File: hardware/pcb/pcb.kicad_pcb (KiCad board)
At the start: 4 copper layers, 41.5 x 61.7 mm, 283 parts, among them J100 Conn_02x05_Odd_Even, J200 Conn_02x05_Odd_Even, J400 AudioJack3_SwitchT, J500 AXT524124, J800 USB_C_Receptacle, SW600 K1-1511SA-02, U1 AXP209, U100 MIMXRT1176DVMAA, U2 SY8008, U200 XC7S25-CSGA225, U201 74LVCH245A, U3 NX3P1108UK, U300 IS66WVC4M16-ALL, U301 MT48H16M32LFB5-6 or IS42VM321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, U302 74LVC1G126, U303 IS66WVC4M16-ALL, U304 74LVC1G126, U4 NX3P1108UK, U400 CS43130, U401 ADP150-1.8, U402 ADP150-1.8, U5 NX3P1108UK, U500 LT3491, U6 NX3P1108UK, U7 ADP121-1.2, U700 W25Q128JVP, U800 USBLC6-2P6, U801 FUSB302UCX, U802 CBTL08GP053, U803 TC358777, X800 19.2MHz, Y100 24MHz, Y101 32.768K, Y400 22.5792MHz

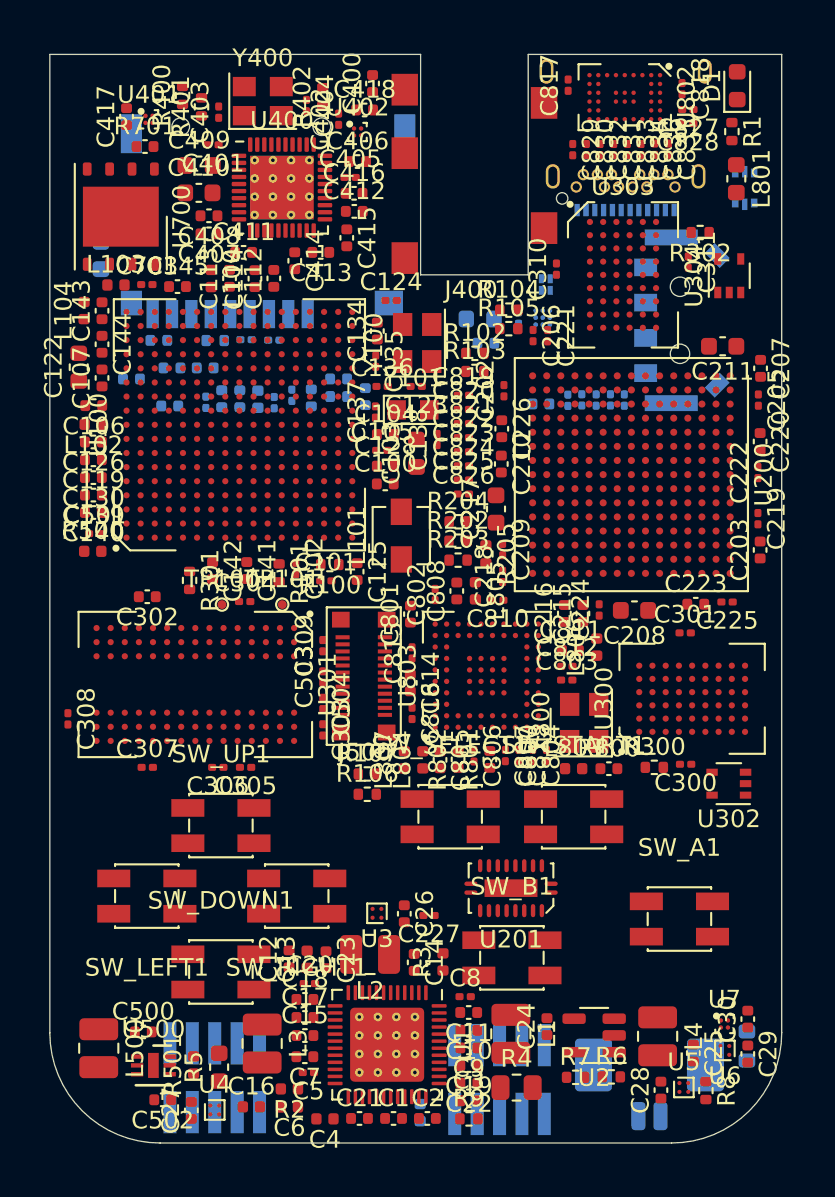
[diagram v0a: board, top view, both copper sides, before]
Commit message: - Working on pcb layout
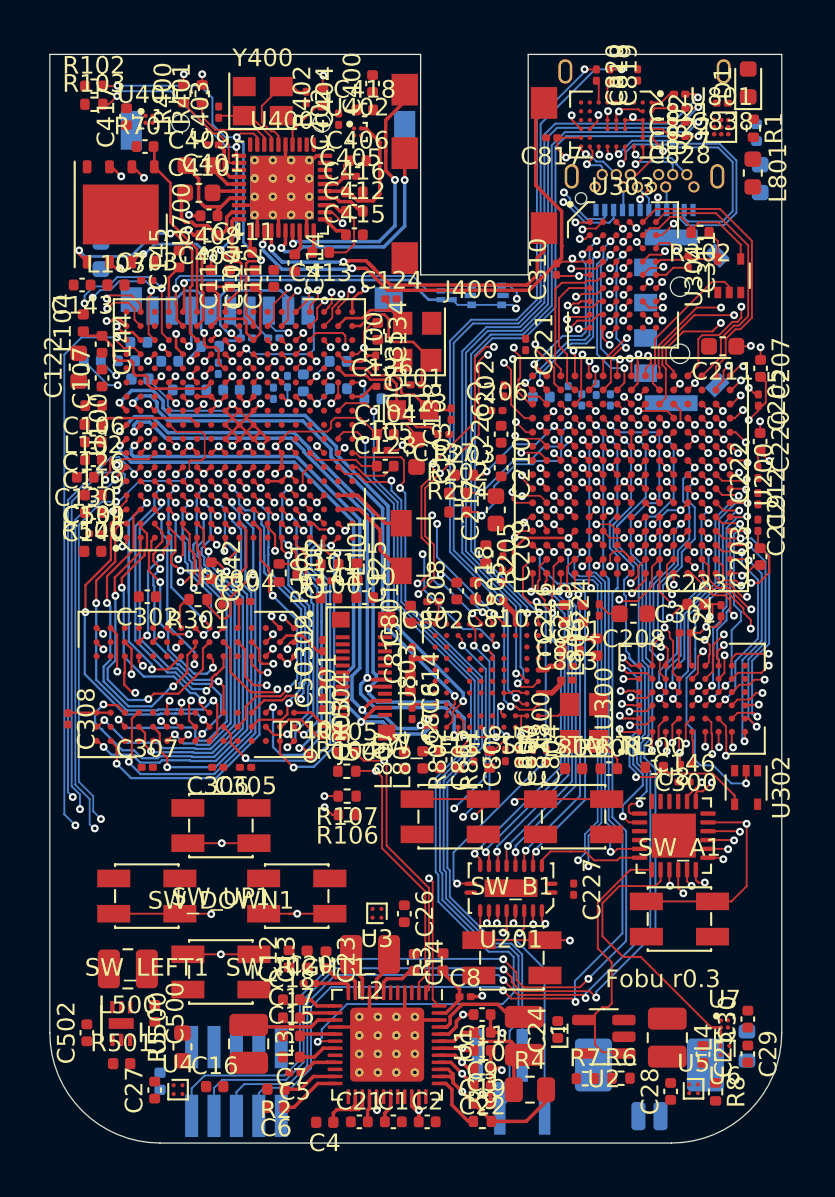
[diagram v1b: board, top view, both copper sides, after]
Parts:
- removed C823, C824, C825, C826, C829, C830, C831, C832, C833, C834, C835, C836: 100nF, Capacitor_SMD:C_0201_0603Metric
- removed J100: Conn_02x05_Odd_Even, Connector_PinHeader_1.27mm:PinHeader_2x05_P1.27mm_Vertical_SMD
- added C146: 100nF, Capacitor_SMD:C_0201_0603Metric, F.Cu at (136.0, 96.0)
- added J101: Conn_01x04, Connector_PinHeader_1.27mm:PinHeader_1x04_P1.27mm_Vertical_SMD_Pin1Left, B.Cu at (126.2, 113.0)
- added U8: PCA9555AHF, Package_DFN_QFN:HVQFN-24-1EP_4x4mm_P0.5mm_EP2.5x2.5mm, F.Cu at (135.4, 99.1)
- C212, C838, U801: moved to F.Cu
- moved R104 27.7 mm to (116.8, 95.4)
- moved R103 26.4 mm to (102.5, 57.6)
- moved R102 26.4 mm to (102.5, 56.6)
- moved R105 25.7 mm to (116.8, 94.4)
- moved C821 22.3 mm to (135.7, 57.0), turned to 180 degrees
- moved C822 22.3 mm to (135.7, 57.8), turned to 180 degrees
- moved C820 20.4 mm to (131.0, 56.0), turned to -90 degrees
- moved C819 20.0 mm to (131.8, 56.0), turned to -90 degrees
- moved C837 19.4 mm to (140.1, 59.2), turned to 90 degrees
- moved L802 17.8 mm to (140.3, 61.8), turned to -90 degrees
- moved C838 16.8 mm to (138.1, 57.5), turned to 180 degrees
- moved U800 15.8 mm to (124.8, 68.4), turned to 0 degrees
- moved J200 14.9 mm to (110.6, 113.0)
- moved R200 14.9 mm to (106.2, 113.0), turned to -90 degrees
- moved U801 14.8 mm to (138.1, 58.9), turned to 0 degrees
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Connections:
- C817 pad 1: +1V8 -> +3V3
- R400 pad 2: SAI4_TX_DATA -> SAI1_RX_SYNC
- R401 pad 2: SAI4_TX_SYNC -> SAI1_RX_BCLK
- R402 pad 2: SAI4_TX_BCLK -> SAI1_RX_DATA0
- U1 pad 6: PMU_VBUSEN -> unconnected-(U1-Pad6)
- U100 pad R5: /mcu/JTAG_TRSTB -> unconnected-(U100-PadR5)
- U100 pad T5: /mcu/JTAG_TDO -> unconnected-(U100-PadT5)
- U100 pad U5: /mcu/JTAG_TDI -> unconnected-(U100-PadU5)
- U200 pad A10: CRAMA_OEN -> CRAMA_A17
- U200 pad A11: CRAMA_CRE -> CRAMA_A15
- U200 pad A12: CRAMA_WAIT -> CRAMA_A13
- U200 pad A14: CRAMA_ADVN -> CRAMA_WAIT
- U200 pad A2: CRAMB_DQ4 -> CRAMB_DQ1
- U200 pad A3: CRAMB_DQ2 -> CRAMB_DQ3
- U200 pad A4: CRAMB_DQ1 -> CRAMB_DQ4
- U200 pad A5: CRAMA_DQ9 -> CRAMA_A20
- U200 pad A6: CRAMA_DQ10 -> CRAMA_A11
- U200 pad A7: CRAMA_DQ6 -> CRAMA_A10
- U200 pad A8: CRAMA_DQ11 -> CRAMA_A9
- U200 pad A9: CRAMA_DQ12 -> CRAMA_ADVN
- U200 pad B1: CRAMB_DQ8 -> CRAMB_A2
- U200 pad B10: CRAMA_LBN -> CRAMA_CEN
- U200 pad B11: CRAMA_CEN -> CRAMA_A14
- U200 pad B12: CRAMA_WEN -> CRAMA_A8
- U200 pad B13: CRAMA_A0 -> CRAMA_A12
- U200 pad B14: CRAMA_A1 -> CRAMA_DQ13
- U200 pad B15: CRAMA_A3 -> CRAMA_DQ15
- U200 pad B2: CRAMB_DQ3 -> CRAMB_DQ2
- U200 pad B5: CRAMB_DQ10 -> CRAMB_DQ7
- U200 pad B9: CRAMA_UBN -> CRAMA_A7
- U200 pad C1: CRAMB_DQ7 -> CRAMB_CRE
- U200 pad C10: CRAMA_DQ15 -> CRAMA_A6
- U200 pad C13: CRAMA_A4 -> CRAMA_A5
- U200 pad C14: CRAMA_A5 -> CRAMA_A19
- U200 pad C15: CRAMA_A2 -> CRAMA_A18
- U200 pad C4: CRAMB_DQ14 -> CRAMB_WEN
- U200 pad C5: CRAMB_DQ9 -> CRAMB_CLK
- U200 pad C6: CRAMA_DQ1 -> CRAMA_DQ7
- U200 pad C7: CRAMA_DQ2 -> CRAMA_WEN
- U200 pad C8: CRAMA_DQ7 -> CRAMA_DQ6
- U200 pad C9: CRAMA_DQ8 -> CRAMA_DQ4
- U200 pad D1: CRAMB_DQ12 -> CRAMB_A0
- U200 pad D10: CRAMA_DQ14 -> CRAMA_DQ1
- U200 pad D11: CRAMA_DQ0 -> CRAMA_DQ2
- U200 pad D12: CRAMA_A6 -> CRAMA_UBN
- U200 pad D13: CRAMA_A7 -> CRAMA_A21
- U200 pad D15: CRAMA_A13 -> CRAMA_DQ14
- U200 pad D2: CRAMB_DQ11 -> CRAMB_A20
- U200 pad D3: CRAMB_OEN -> unconnected-(U200-PadD3)
- U200 pad D4: CRAMB_DQ13 -> CRAMB_ADVN
- U200 pad D7: CRAMA_DQ3 -> CRAMA_DQ0
- U200 pad D8: CRAMA_DQ4 -> CRAMA_DQ3
- U200 pad D9: CRAMA_DQ13 -> CRAMA_A16
- U200 pad E1: CRAMB_LBN -> CRAMB_A1
- U200 pad E11: CRAMA_A9 -> CRAMA_OEN
- U200 pad E12: CRAMA_A10 -> CRAMA_A3
- U200 pad E13: CRAMA_A11 -> CRAMA_A0
- U200 pad E14: CRAMA_A12 -> CRAMA_DQ11
- U200 pad E15: CRAMA_A17 -> CRAMA_DQ12
- U200 pad E2: CRAMB_DQ15 -> CRAMB_A11
- U200 pad E3: CRAMB_UBN -> CRAMB_A10
- U200 pad F1: CRAMB_WEN -> CRAMB_A4
- U200 pad F11: CRAMA_A8 -> CRAMA_A4
- U200 pad F14: CRAMA_A16 -> CRAMA_DQ8
- U200 pad F15: CRAMA_A15 -> CRAMA_DQ9
- U200 pad F3: CRAMB_WAIT -> CRAMB_DQ0
- U200 pad F4: CRAMB_CRE -> CRAMB_A9
- U200 pad G1: CRAMB_ADVN -> CRAMB_A7
- U200 pad G11: CRAMA_A20 -> CRAMA_CRE
- U200 pad G12: CRAMA_A21 -> CRAMA_A1
- U200 pad G13: CRAMA_A18 -> CRAMA_A2
- U200 pad G14: CRAMA_A19 -> CRAMA_DQ10
- U200 pad G15: CRAMA_A14 -> CRAMA_LBN
- U200 pad G4: CRAMB_DQ0 -> CRAMB_WAIT
- U200 pad H1: CRAMB_CLK -> CRAMB_A16
- U200 pad H2: CRAMB_A3 -> CRAMB_A17
- U200 pad H3: CRAMB_A1 -> CRAMB_A8
- U200 pad H4: CRAMB_A0 -> CRAMB_A18
- U200 pad J1: CRAMB_A7 -> CRAMB_A5
- U200 pad J2: CRAMB_A2 -> CRAMB_A3
- U200 pad J3: CRAMB_A5 -> CRAMB_A19
- U200 pad J4: CRAMB_A4 -> CRAMB_DQ15
- U200 pad K1: CRAMB_A6 -> CRAMB_A21
- U200 pad K14: unconnected-(U200-PadK14) -> SAI4_TX_BCLK
- U200 pad K2: CRAMB_A9 -> CRAMB_A6
- U200 pad K3: CRAMB_A8 -> unconnected-(U200-PadK3)
- U200 pad L1: CRAMB_A11 -> CRAMB_A13
- U200 pad L14: unconnected-(U200-PadL14) -> SAI4_TX_SYNC
- U200 pad L15: unconnected-(U200-PadL15) -> SAI4_TX_DATA
- U200 pad M1: CRAMB_A10 -> CRAMB_A15
- U200 pad M10: CSI_D1 -> CSI_D8
- U200 pad M13: unconnected-(U200-PadM13) -> UART2_RXD
- U200 pad M14: /fpga/K_UP -> /fpga/K_RIGHT
- U200 pad M2: CRAMB_A15 -> CRAMB_DQ14
- U200 pad M3: CRAMB_A13 -> CRAMB_A12
- U200 pad M4: CRAMB_A12 -> CRAMB_DQ13
- U200 pad M8: CSI_D13 -> CSI_D10
- U200 pad M9: CSI_D0 -> CSI_D6
- U200 pad N1: CRAMB_A19 -> CRAMB_DQ12
- U200 pad N10: CSI_D4 -> CSI_VSYNC
- U200 pad N11: CSI_D5 -> CSI_D15
- U200 pad N12: CSI_D2 -> CSI_D5
- U200 pad N13: unconnected-(U200-PadN13) -> UART2_TXD
- U200 pad N14: /fpga/K_RIGHT -> /fpga/K_SELECT
- U200 pad N15: /fpga/K_DOWN -> /fpga/K_UP
- U200 pad N2: CRAMB_A14 -> CRAMB_DQ11
- U200 pad N3: CRAMB_A17 -> CRAMB_A14
- U200 pad N7: CSI_D15 -> CSI_D11
- U200 pad P1: CRAMB_A18 -> CRAMB_DQ9
- U200 pad P10: CSI_D6 -> CSI_D13
- U200 pad P11: CSI_D7 -> CSI_D0
- U200 pad P12: CSI_D3 -> CSI_D4
- U200 pad P14: /fpga/K_START -> /fpga/K_A
- U200 pad P15: /fpga/K_SELECT -> /fpga/K_START
- U200 pad P2: unconnected-(U200-PadP2) -> CRAMB_DQ10
- U200 pad P3: CRAMB_A16 -> CRAMB_DQ8
- U200 pad P6: CSI_PCLK -> CSI_D9
- U200 pad P7: CSI_VSYNC -> CSI_D7
- U200 pad R10: CSI_D9 -> CSI_HSYNC
- U200 pad R11: CSI_D10 -> CSI_D3
- U200 pad R12: CSI_D11 -> CSI_D2
- U200 pad R13: /fpga/K_A -> /fpga/K_DOWN
- U200 pad R2: unconnected-(U200-PadR2) -> CRAMB_UBN
- U200 pad R3: CRAMB_A21 -> CRAMB_OEN
- U200 pad R4: CRAMB_A20 -> CRAMB_LBN
- U200 pad R5: CSI_HSYNC -> CSI_PCLK
- U200 pad R9: CSI_D8 -> CSI_D1
- U201 pad 15: /fpga/K_DOWN -> /fpga/K_UP
- U201 pad 18: /fpga/K_UP -> /fpga/K_DOWN
- U201 pad 2: KEY_UP -> KEY_DOWN
- U201 pad 5: KEY_DOWN -> KEY_UP
- U302 pad 2: CRAM_CEN -> CRAMA_CEN
- U802 pad B1: Net-(C824-Pad2) -> GND
- U802 pad B6: Net-(C835-Pad1) -> /usb/TYPEC_TX2N
- U802 pad C1: Net-(C823-Pad2) -> GND
- U802 pad C6: Net-(C836-Pad1) -> /usb/TYPEC_TX2P
- U802 pad D6: Net-(C834-Pad1) -> /usb/TYPEC_RX2P
- U802 pad E4: +1V8 -> +3V3
- U802 pad E6: Net-(C833-Pad1) -> /usb/TYPEC_RX2N
- U802 pad F6: Net-(C831-Pad1) -> /usb/TYPEC_TX1N
- U802 pad G6: Net-(C832-Pad1) -> /usb/TYPEC_TX1P
- U802 pad H1: Net-(C825-Pad2) -> GND
- U802 pad H3: +1V8 -> +3V3
- U802 pad H4: I2C1_SDA -> I2C3_SCL
- U802 pad H6: Net-(C830-Pad1) -> /usb/TYPEC_RX1P
- U802 pad J1: Net-(C826-Pad2) -> GND
- U802 pad J4: I2C1_SCL -> I2C3_SDA
- U802 pad J5: +1V8 -> +3V3
- U802 pad J6: Net-(C829-Pad1) -> /usb/TYPEC_RX1N
- U803 pad J7: Net-(C823-Pad1) -> unconnected-(U803-PadJ7)
- U803 pad J9: Net-(C825-Pad1) -> unconnected-(U803-PadJ9)
- U803 pad K7: Net-(C824-Pad1) -> unconnected-(U803-PadK7)
- U803 pad K9: Net-(C826-Pad1) -> unconnected-(U803-PadK9)
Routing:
- net GND: track 0.00 -> 160.6 mm, vias 0 -> 76
- net I2C1_SCL: track 0.00 -> 102.6 mm, vias 0 -> 4
- net I2C1_SDA: track 0.00 -> 97.8 mm, vias 0 -> 4
- net I2C3_SCL: track 0.00 -> 78.1 mm, vias 0 -> 6
- net UART2_TXD: track 0.00 -> 78.0 mm, vias 0 -> 5
- net I2C3_SDA: track 0.00 -> 77.1 mm, vias 0 -> 6
- net UART2_RXD: track 0.00 -> 71.3 mm, vias 0 -> 4
- net /fpga/FPGA_TDO: track 0.00 -> 65.4 mm, vias 0 -> 3
- net /fpga/FPGA_TCK: track 0.00 -> 64.3 mm, vias 0 -> 3
- net /fpga/FPGA_TMS: track 0.00 -> 63.5 mm, vias 0 -> 3
- net FSPI_2A_SCK: track 0.00 -> 61.0 mm, vias 0 -> 4
- net PMU_IRQ: track 0.00 -> 61.0 mm, vias 0 -> 3
- net /fpga/FPGA_TDI: track 0.00 -> 59.9 mm, vias 0 -> 3
- net I2C4_SDA: track 0.00 -> 58.4 mm, vias 0 -> 5
- net I2C4_SCL: track 0.00 -> 56.6 mm, vias 0 -> 5
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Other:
- copper layers 4 -> 6
- board text added: "Fobu r0.3"
